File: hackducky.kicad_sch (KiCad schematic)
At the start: 49 parts, among them J1 USB_A, J2 Conn_02x02_Top_Bottom, J3 Micro_SD_Card, P2 USB_C_Plug, SW2 SW_DIP_x04, SW3 BOOT_SEL, U1 W25Q16JVSS, U2 AP2112K-3.3, U3 USBLC6-2P6, U4 RP2040, U5 USBLC6-2P6, Y1 Crystal_GND24

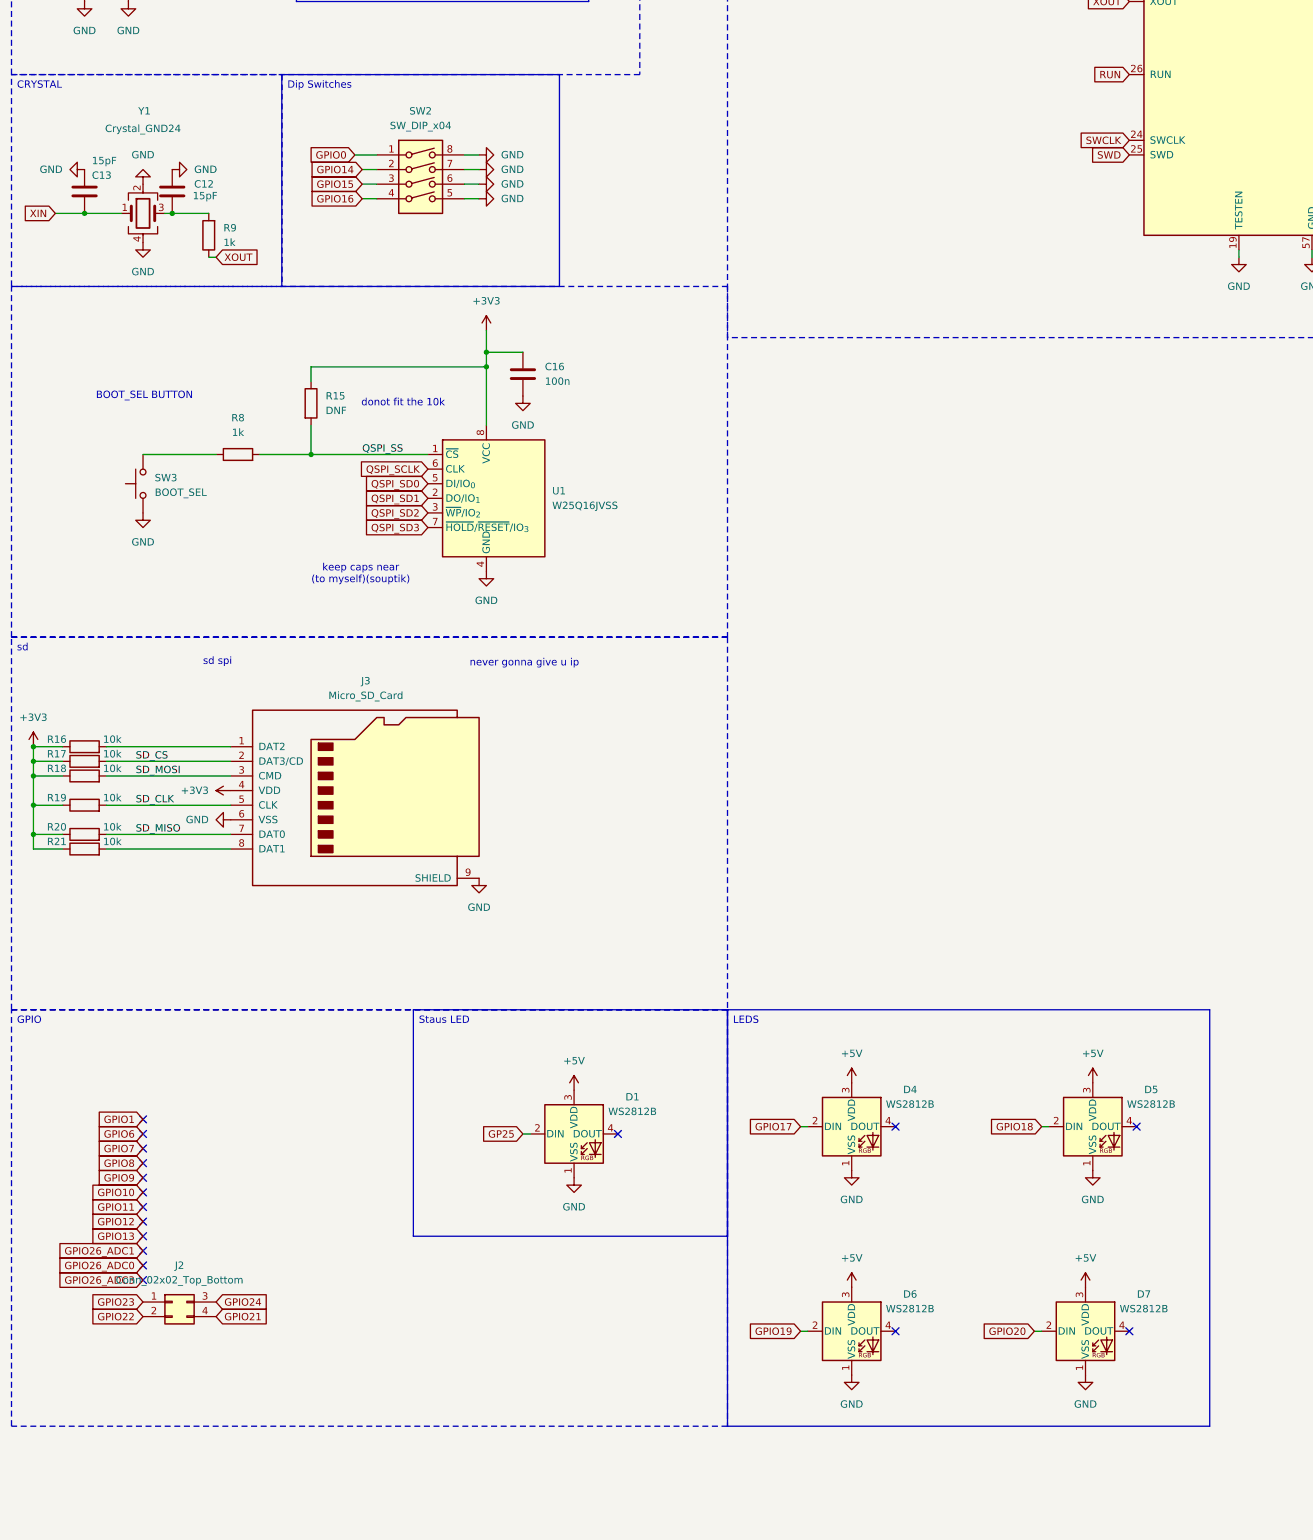
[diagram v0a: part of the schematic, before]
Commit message: full done yayayay
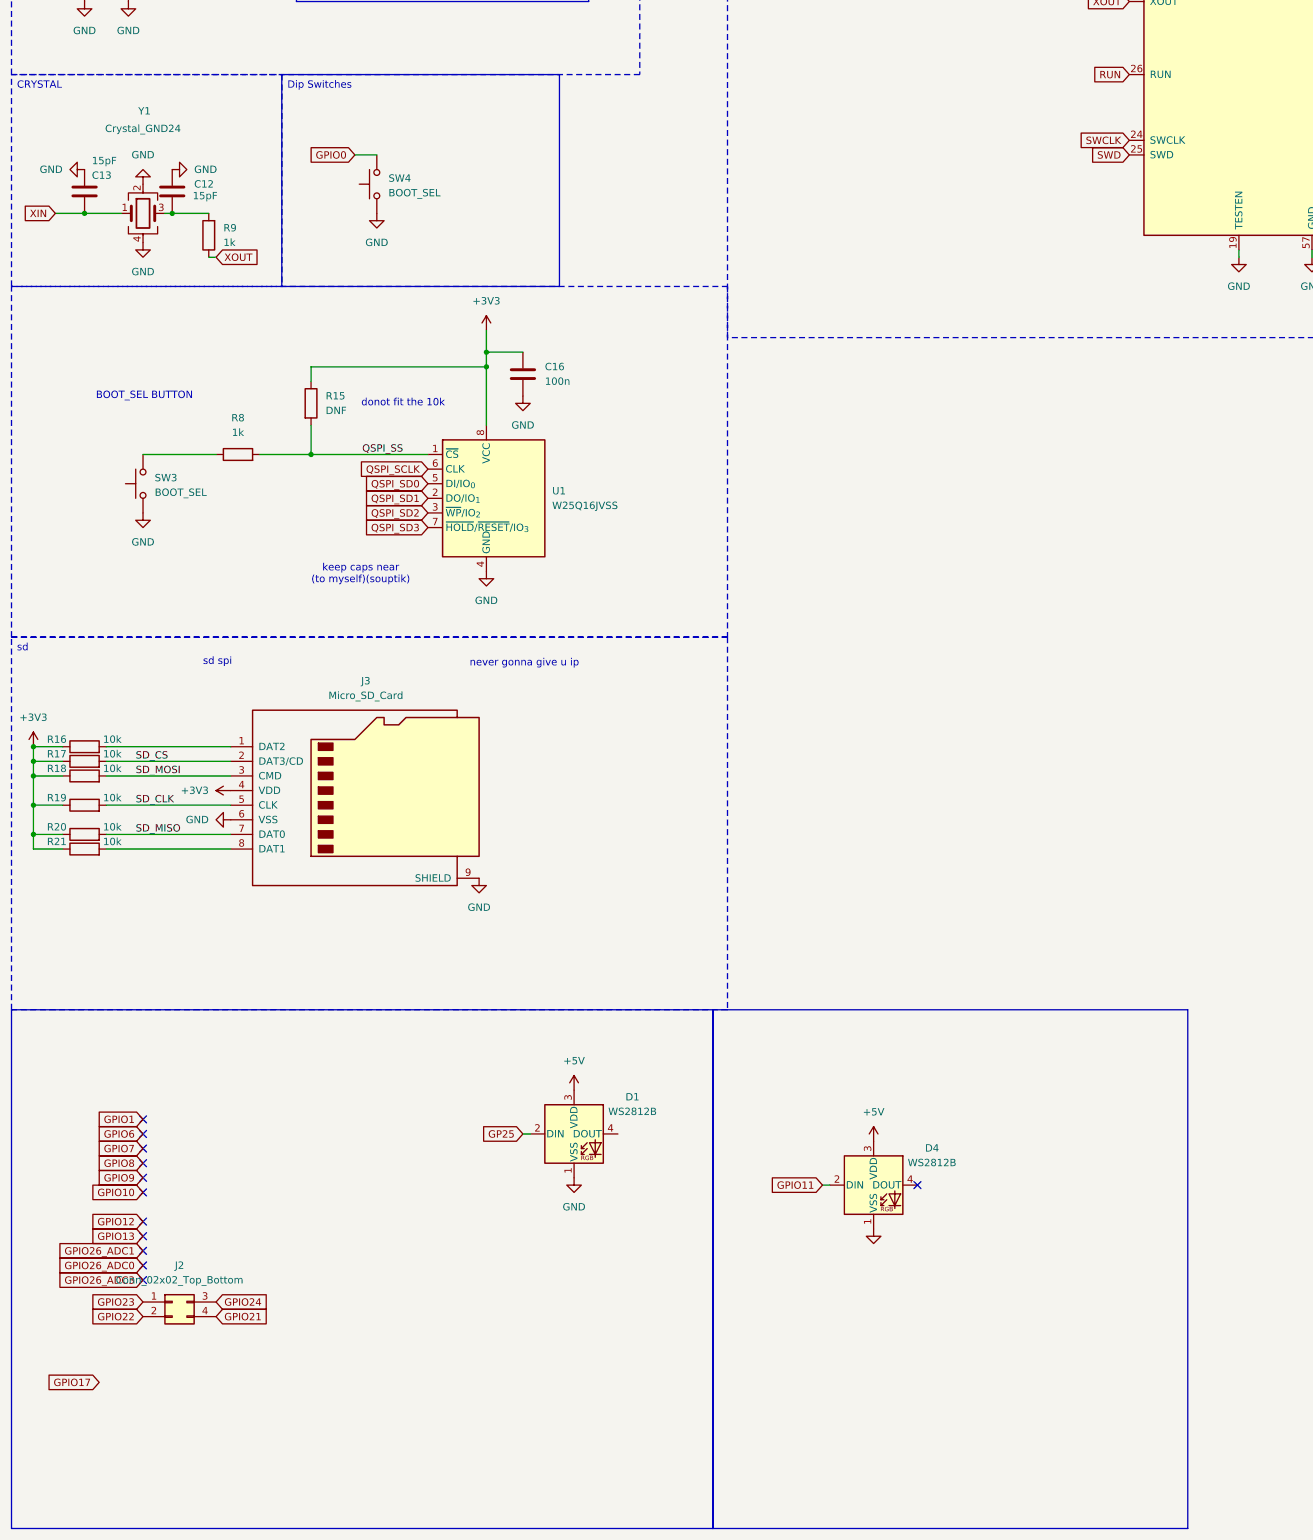
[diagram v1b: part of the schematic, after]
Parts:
- removed D5, D6, D7: WS2812B, LED_SMD:LED_WS2812B-2020_PLCC4_2.0x2.0mm, symbol LED:SK6812
- removed SW2: SW_DIP_x04, Button_Switch_THT:SW_DIP_SPSTx04_Slide_6.7x11.72mm_W7.62mm_P2.54mm_LowProfile, symbol Switch:SW_DIP_x04
- added SW4: BOOT_SEL, Button_Switch_SMD:SW_Push_SPST_NO_Alps_SKRK, symbol Switch:SW_Push
- SW3: footprint Button_Switch_SMD:SW_Push_1P1T_XKB_TS-1187A -> Button_Switch_SMD:SW_Push_SPST_NO_Alps_SKRK
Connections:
- net GND: now also SW4.1
- net GPIO0: now also SW4.2
- net GPIO11: now also D4.2 (DIN)
- net GPIO17: no longer D4.2 (DIN)
- no-connect marks 27 -> 22
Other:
- moved on the sheet: D4
